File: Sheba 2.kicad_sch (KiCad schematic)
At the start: 66 parts, among them J2 Conn_01x03_Pin, J3 Conn_01x03_Pin, J4 Conn_01x03_Pin, J7 Conn_01x06_Pin, J8 Conn_01x02_Pin, J9 Conn_02x04_Top_Bottom, P1 USB_C_Plug_USB2.0, SW1 SW_SPDT, U1 AP62300TWU, U3 MIC5504-3.3YM5, U4 STM32F072CBTx

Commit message: Actually get ready to add protections
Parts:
- removed Battery1: XT-60, Connector_AMASS:AMASS_XT60-F_1x02_P7.20mm_Vertical, symbol Device:Battery
- removed C1, C15: C0.1uF, Capacitor_SMD:C_1206_3216Metric_Pad1.33x1.80mm_HandSolder, symbol Device:C_Small
- removed C10, C12, C16, C18, C3, C5, C6, C7: C1uF, Capacitor_SMD:C_1206_3216Metric_Pad1.33x1.80mm_HandSolder, symbol Device:C_Small
- removed C11: C2.2uF, Capacitor_SMD:C_1206_3216Metric_Pad1.33x1.80mm_HandSolder, symbol Device:C_Small
- removed C13, C19: C22uF, Capacitor_SMD:C_1206_3216Metric_Pad1.33x1.80mm_HandSolder, symbol Device:C_Small
- removed C8: C10uF, Capacitor_SMD:C_1206_3216Metric_Pad1.33x1.80mm_HandSolder, symbol Device:C_Small
- removed C9: C0.01uF, Capacitor_SMD:C_1206_3216Metric_Pad1.33x1.80mm_HandSolder, symbol Device:C_Small
- removed D2, D4, D6, D7, D8: LED Green, LED_SMD:LED_1206_3216Metric_Pad1.42x1.75mm_HandSolder, symbol Device:LED
- removed D3, D5: LED Red, LED_SMD:LED_1206_3216Metric_Pad1.42x1.75mm_HandSolder, symbol Device:LED
- removed H1, H2, H3, H4: MountingHole_Pad, MountingHole:MountingHole_2.2mm_M2_DIN965_Pad, symbol Mechanical:MountingHole_Pad
- removed J2, J3, J4: Conn_01x03_Pin, Connector_PinSocket_2.54mm:PinSocket_1x03_P2.54mm_Vertical, symbol Connector:Conn_01x03_Pin
- removed L1: L3.3uH, Inductor_SMD:L_1206_3216Metric, symbol Device:L
- removed MD1, MD2, MD3: ZXBM5210-S, Package_SO:SOIC-8_3.9x4.9mm_P1.27mm, symbol Driver_Motor:ZXBM5210-S
- removed MT1: ICM-42670-P, Library:XDCR_ICM-42670-P, symbol ICM-42670-P:ICM-42670-P
- removed Motor Terminal1: 6x Motor Port, TerminalBlock_4Ucon:TerminalBlock_4Ucon_1x06_P3.50mm_Horizontal, symbol Connector:Screw_Terminal_01x06
- removed R10, R11, R12, R13, R6, R7, R8, R9: R220, Resistor_SMD:R_1206_3216Metric_Pad1.30x1.75mm_HandSolder, symbol Device:R
- removed R2, R4, R5: R10k, Resistor_SMD:R_1206_3216Metric_Pad1.30x1.75mm_HandSolder, symbol Device:R
- removed U1: AP62300TWU, Package_TO_SOT_SMD:TSOT-23-6_HandSoldering, symbol Regulator_Switching:AP62300TWU
- removed U3: MIC5504-3.3YM5, Package_TO_SOT_SMD:SOT-23-5_HandSoldering, symbol Regulator_Linear:MIC5504-3.3YM5
- D1: value LED Red -> LED Green; DigiKey 150120RS75000 -> 150120VS75000
- J1: renamed from J8; footprint Connector_PinHeader_2.54mm:PinHeader_1x02_P2.54mm_Vertical -> Connector_PinHeader_2.54mm:PinHeader_1x03_P2.54mm_Vertical; symbol Connector:Conn_01x02_Pin -> Connector:Conn_01x03_Pin
- R3: value R56.2k -> R220; DigiKey CRCW120652K3FKEA -> RMCF1206JT220R
- renumbered C2 to C1, C4 to C2, C14 to C3, C17 to C4, EP3 to EP1, EP1 to EP2, EP2 to EP3, J9 to J2, J7 to J3, R14 to R1, R1 to R2, U4 to U1
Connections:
- net +5V: no longer R3.1
- net BLINKY: now also R3.1
- net GND: now also D1.1 (K), J1.1 (Pin_1)
- net M3_REV: no longer D1.2 (A)
- net USART3_TX: now also J1.3 (Pin_3); no longer J1.1 (Pin_1)
- net at R3.2: now also D1.2 (A)
- net I2C2_SCL: no longer names the net of U1.26 (PB13)
- net I2C2_SDA: no longer names the net of U1.27 (PB14)
- net IMU_INT: no longer names the net of U1.28 (PB15)
- no-connect marks 12 -> 9
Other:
- added sheet Power & Motors (Power & Motors.kicad_sch)
- note added: "CPU STATUS LED"
- note added: "Kiwi/Differential Drive Switch"
- note removed: "12V to 5V"
- note removed: "3V3 LDO Power Supply"
- note removed: "AP_CS wired to VDD for I2C mode"
- note removed: "I2C Pull-ups"
- note removed: "IMU - Accel/Gyro/Temp chip ICM-42670-P"
- note removed: "Indicator LEDs"
- note removed: "Motor Controllers"
- note removed: "Servo Ports"
- note removed: "VIN: 4.2 to 18V"
- note removed: "VREF is wired to VDD to enable PWM control"
- moved on the sheet: C1, C2, C3, C4, EP1, EP2, EP3, J2, J3, P1, R1, R2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

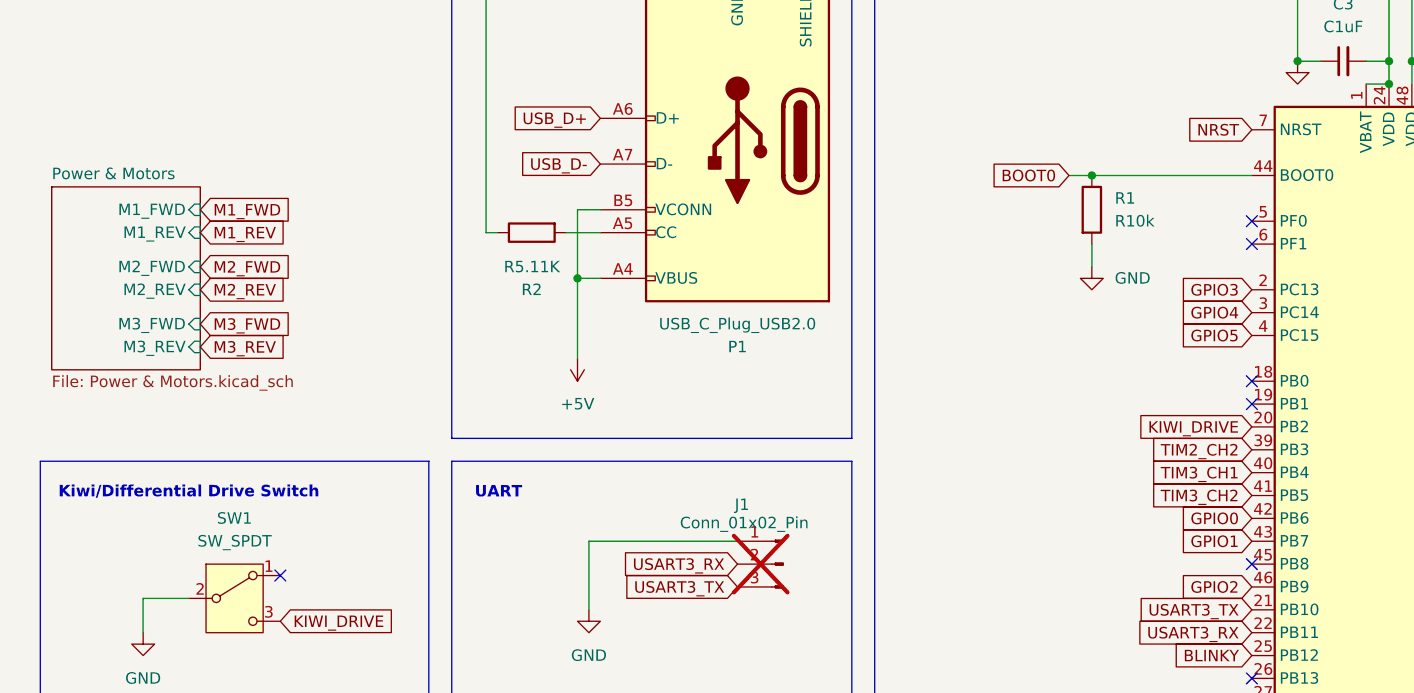
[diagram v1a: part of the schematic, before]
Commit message: Ready to finalize Rev3
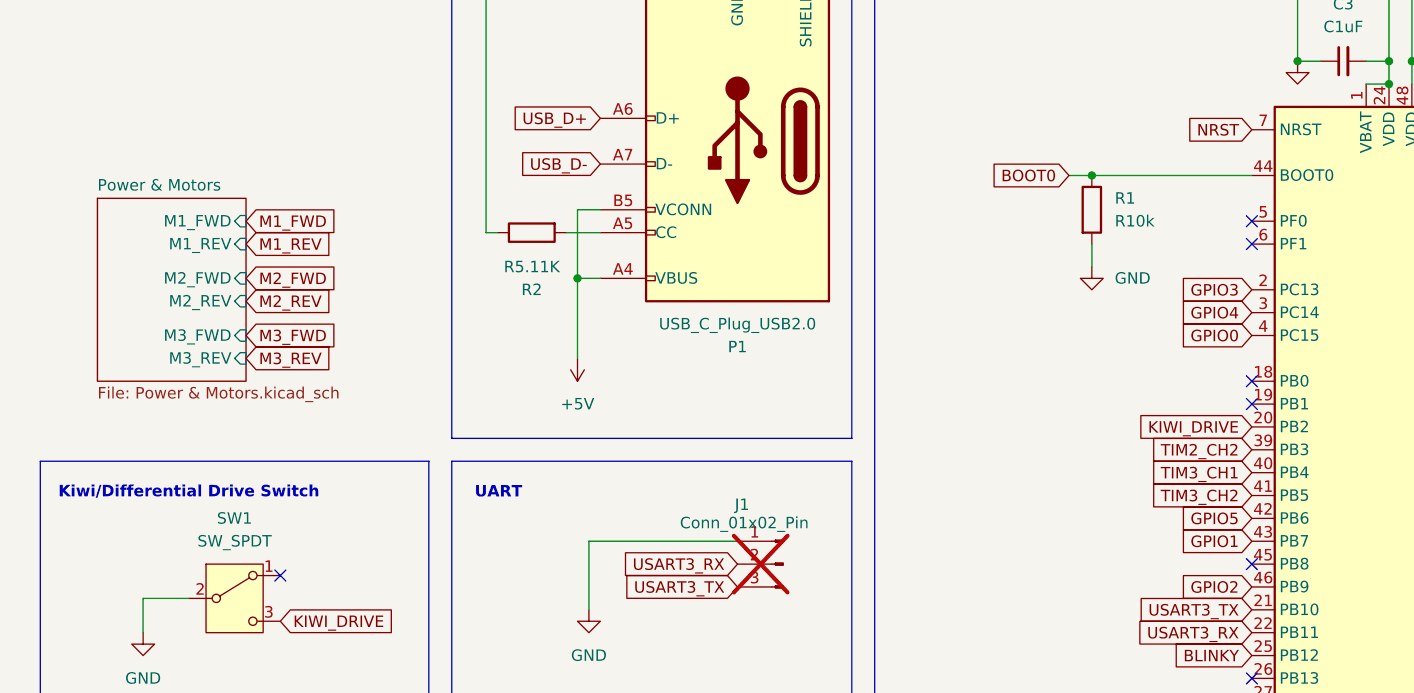
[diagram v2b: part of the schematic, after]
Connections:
- net GPIO0: now also U1.4 (PC15); no longer U1.42 (PB6)
- net GPIO5: now also U1.42 (PB6); no longer U1.4 (PC15)
